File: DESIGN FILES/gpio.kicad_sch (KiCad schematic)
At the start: 20 parts, among them U401 MIMXRT1064CVL5B

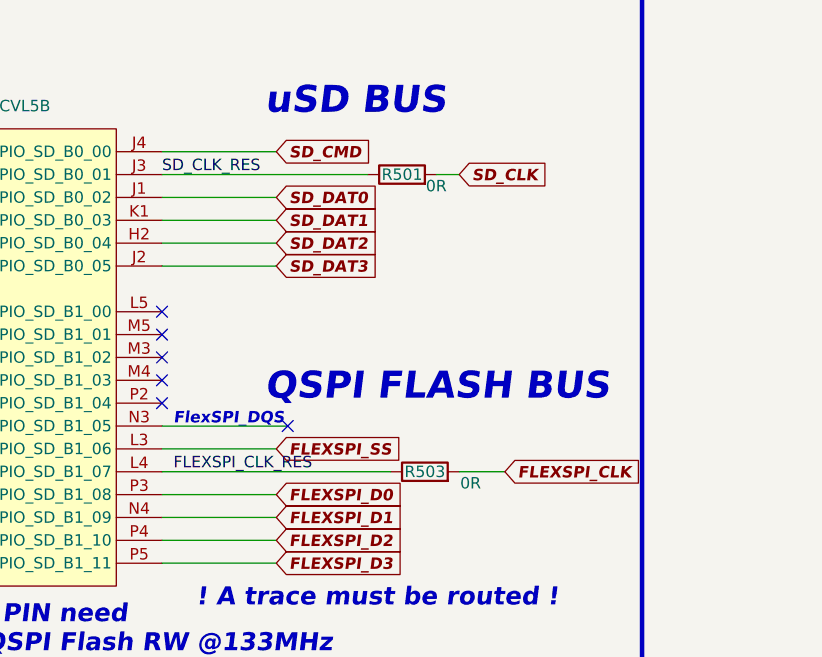
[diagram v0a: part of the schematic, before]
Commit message: updates
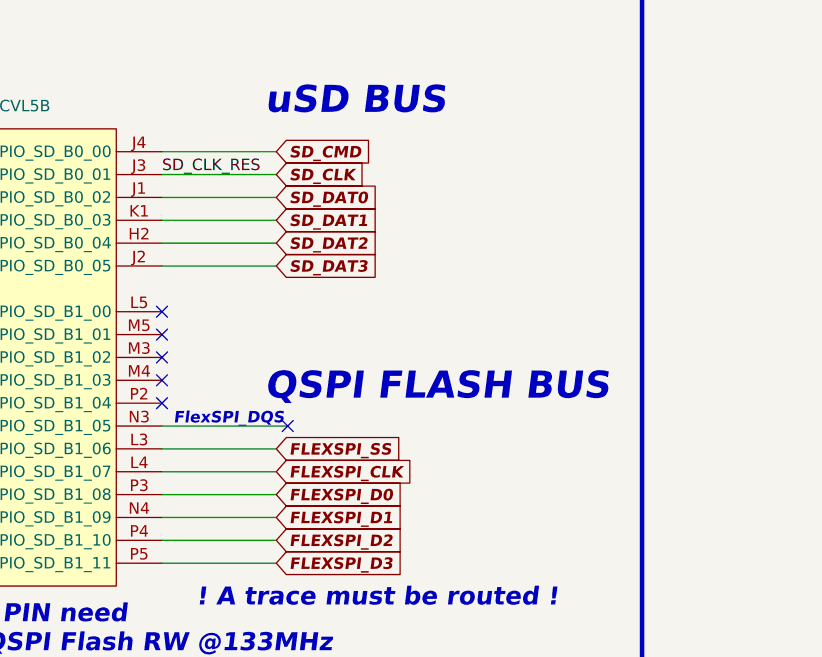
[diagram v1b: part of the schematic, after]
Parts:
- removed R501, R503: 0R, MY RESISTOR LIBRARY:0603WAF0000T5E, symbol MY RESISTOR LIBRARY:0603WAF0000T5E
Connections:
- net FLEXSPI_CLK_RES is gone; now on net FLEXSPI_CLK: U401.L4 (GPIO_SD_B1_07)
- net SD_CLK_RES is gone; now on net SD_CLK: U401.J3 (GPIO_SD_B0_01)
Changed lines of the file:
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@@
-    (stroke (width 0) (type default) (color 0 0 0 0))
-  )
-  (wire (pts (xy 132.08 247.65) (xy 157.48 247.65))
     (stroke (width 0) (type default) (color 0 0 0 0))
   )
@@
     (stroke (width 0) (type default) (color 0 0 0 0))
   )
-  (wire (pts (xy 162.56 214.63) (xy 165.1 214.63))
-    (stroke (width 0) (type default) (color 0 0 0 0))
-  )
   (wire (pts (xy 335.28 91.44) (xy 347.98 91.44))
     (stroke (width 0) (type default) (color 0 0 0 0))
@@
     (stroke (width 0.5) (type default) (color 0 0 0 0))
   )
+  (wire (pts (xy 132.08 214.63) (xy 144.78 214.63))
+    (stroke (width 0) (type default) (color 0 0 0 0))
+  )
   (wire (pts (xy 229.87 78.74) (xy 229.87 81.28))
     (stroke (width 0) (type default) (color 0 0 0 0))
@@
     (stroke (width 0) (type default) (color 0 0 0 0))
   )
-  (wire (pts (xy 132.08 214.63) (xy 154.94 214.63))
-    (stroke (width 0) (type default) (color 0 0 0 0))
-  )
   (wire (pts (xy 85.09 57.15) (xy 87.63 57.15))
     (stroke (width 0) (type default) (color 0 0 0 0))
@@
     (stroke (width 0) (type default) (color 0 0 0 0))
   )
-  (wire (pts (xy 170.18 247.65) (xy 165.1 247.65))
+  (wire (pts (xy 132.08 247.65) (xy 144.78 247.65))
     (stroke (width 0) (type default) (color 0 0 0 0))
   )
@@
   (text "JTAG_MOD : GND for normal operation" (at 226.06 96.52 0)
     (effects (font (size 1.27 1.27) bold italic) (justify left bottom))
-  )
-  (label "FLEXSPI_CLK_RES" (at 133.35 247.65 0)
-    (effects (font (size 1.27 1.27)) (justify left bottom))
   )
   (label "I2S_BCLK_RES" (at 275.59 154.94 0)
@@
     )
   )
-  (global_label "FLEXSPI_CLK" (shape input) (at 170.18 247.65 0) (fields_autoplaced)
-    (effects (font (size 1.27 1.27) (thickness 0.254) bold italic) (justify left))
-    (property "Intersheet References" "${INTERSHEET_REFS}" (id 0) (at 185.1343 247.523 0)
+  (global_label "FLEXSPI_CLK" (shape input) (at 144.78 247.65 0) (fields_autoplaced)
+    (effects (font (size 1.27 1.27) (thickness 0.254) bold italic) (justify left))
+    (property "Intersheet References" "${INTERSHEET_REFS}" (id 0) (at 159.7343 247.523 0)
       (effects (font (size 1.27 1.27) (thickness 0.254) bold italic) (justify left) hide)
     )
@@
     )
   )
-  (global_label "SD_CLK" (shape input) (at 165.1 214.63 0) (fields_autoplaced)
-    (effects (font (size 1.27 1.27) bold italic) (justify left))
-    (property "Intersheet References" "${INTERSHEET_REFS}" (id 0) (at 174.9743 214.757 0)
+  (global_label "SD_CLK" (shape input) (at 144.78 214.63 0) (fields_autoplaced)
+    (effects (font (size 1.27 1.27) bold italic) (justify left))
+    (property "Intersheet References" "${INTERSHEET_REFS}" (id 0) (at 154.6543 214.757 0)
       (effects (font (size 1.27 1.27) bold italic) (justify left) hide)
     )
@@
     (pin "P5")
   )
-  (symbol (lib_id "MY RESISTOR LIBRARY:0603WAF0000T5E") (at 161.29 247.65 90) (unit 1)
-    (in_bom yes) (on_board yes)
-    (property "Reference" "R503" (id 0) (at 161.29 247.65 90))
-    (property "Value" "0R" (id 1) (at 166.37 248.92 90))
-    (property "Footprint" "MY RESISTOR LIBRARY:0603WAF0000T5E" (id 2) (at 161.29 249.428 90)
-      (effects (font (size 1.27 1.27)) hide)
-    )
-    (property "Datasheet" "~" (id 3) (at 161.29 247.65 0)
-      (effects (font (size 1.27 1.27)) hide)
-    )
-    (pin "1")
-    (pin "2")
-  )
   (symbol (lib_id "MY CAPACITOR LIBRARY:CL05B104KB54PNC") (at 254 72.39 0) (unit 1)
     (in_bom yes) (on_board yes) (fields_autoplaced)
@@
     (pin "1")
   )
-  (symbol (lib_id "MY RESISTOR LIBRARY:0603WAF0000T5E") (at 158.75 214.63 90) (unit 1)
-    (in_bom yes) (on_board yes)
-    (property "Reference" "R501" (id 0) (at 158.75 214.63 90))
-    (property "Value" "0R" (id 1) (at 162.56 215.9 90))
-    (property "Footprint" "MY RESISTOR LIBRARY:0603WAF0000T5E" (id 2) (at 158.75 216.408 90)
-      (effects (font (size 1.27 1.27)) hide)
-    )
-    (property "Datasheet" "~" (id 3) (at 158.75 214.63 0)
-      (effects (font (size 1.27 1.27)) hide)
-    )
-    (pin "1")
-    (pin "2")
-  )
   (symbol (lib_id "MY RESISTOR LIBRARY:0603WAF0000T5E") (at 265.43 142.24 90) (unit 1)
